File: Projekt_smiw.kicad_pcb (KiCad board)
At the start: 4 copper layers, 53 x 33 mm, 24 parts, among them J1 USB_C_Receptacle_USB2.0, J2 Conn_01x08, J3 Conn_01x10, SW1 SW_Omron_B3FS, SW2 SW_Omron_B3FS, U1 USBLC6-2P6, U2 NCP1117-3.3_SOT223, U4 ESP32-S3-PICO-1

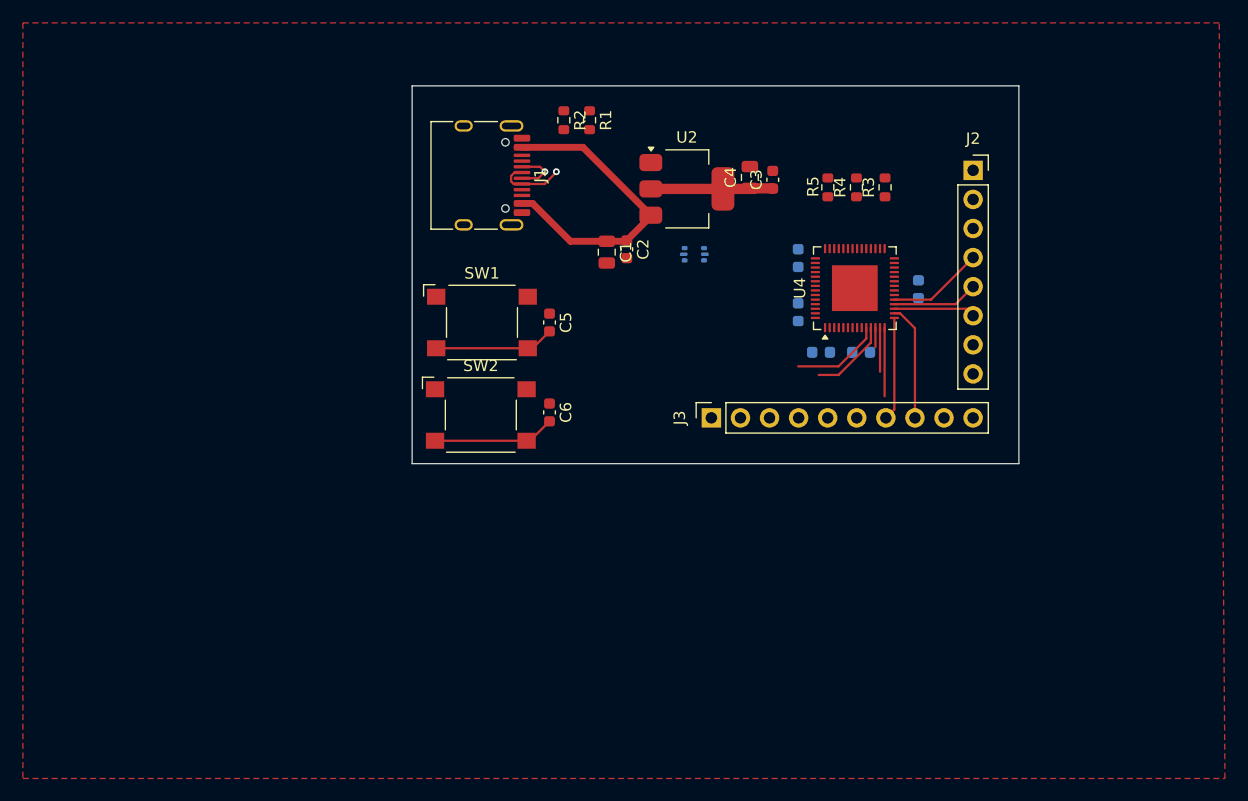
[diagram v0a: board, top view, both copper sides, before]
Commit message: pvcv1
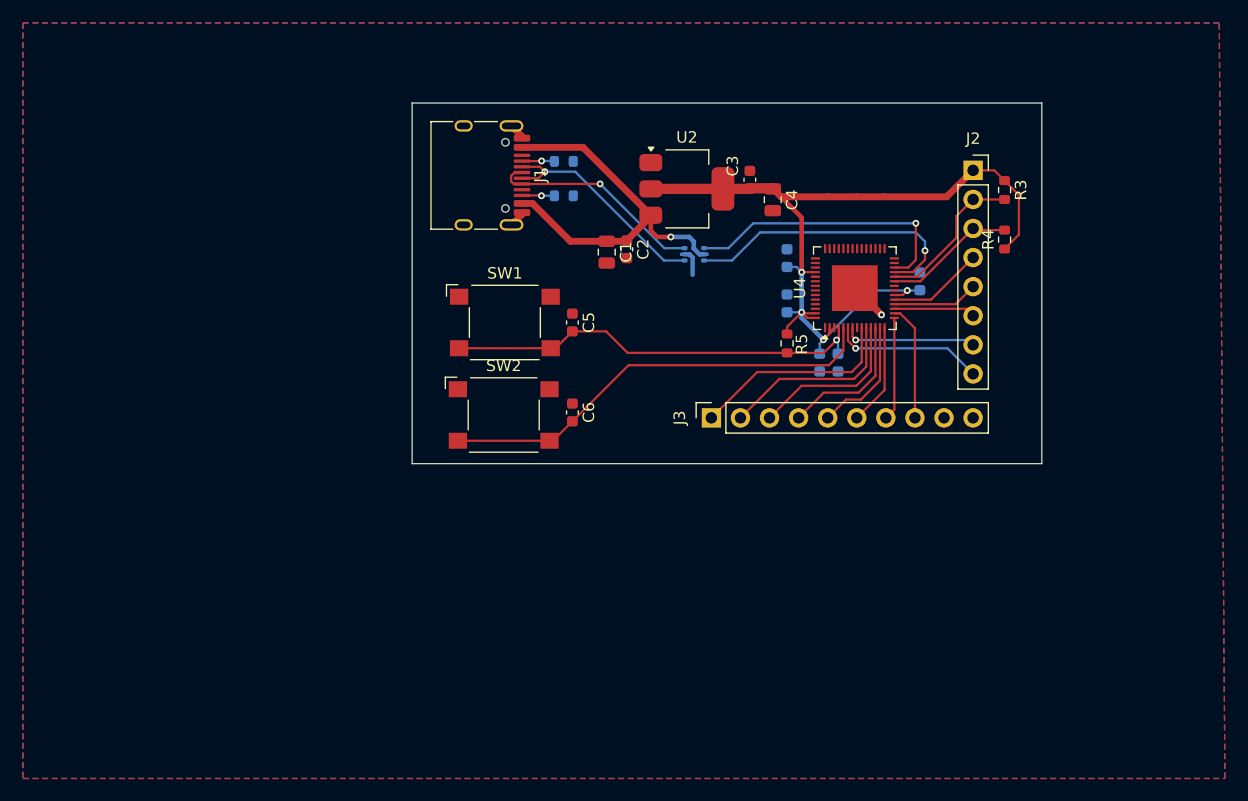
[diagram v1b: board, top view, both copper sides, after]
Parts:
- R1, R2: moved to B.Cu
- moved R5 14.1 mm to (195.8, 62.5), turned to -90 degrees
- moved R4 13.7 mm to (214.8, 53.4)
- moved R3 10.4 mm to (214.8, 49.1), turned to -90 degrees
- moved R1 6.97 mm to (176.2, 49.6), turned to 180 degrees
- moved R2 3.60 mm to (176.2, 46.6), turned to 180 degrees
- moved C4 2.79 mm to (194.5, 50.0), turned to -90 degrees
- moved C7 2.21 mm to (200.2, 64.2), turned to 90 degrees
- moved C3 2.00 mm to (192.5, 48.2)
- moved C5 2.00 mm to (177.0, 60.7)
- moved C6 2.00 mm to (177.0, 68.5)
- moved SW1 2.00 mm to (171.1, 60.7)
- moved SW2 2.00 mm to (171.0, 68.8)
- moved C9 1.24 mm to (195.8, 59.0)
- moved C8 0.97 mm to (195.8, 55.0)
- moved C10 0.91 mm to (198.6, 64.2), turned to -90 degrees
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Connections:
- J2 pad 2: /CS BME280 -> /SCL
- J2 pad 3: /CS FRAM SPI -> /SDA
- J2 pad 7: /SDA -> /CS BME280
- J2 pad 8: /SCL -> /CS FRAM SPI
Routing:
- net +3.3V: track 10.7 -> 77.3 mm, vias 0 -> 4
- net /BOOT: track 10.7 -> 38.9 mm
- net /RESET: track 10.5 -> 37.2 mm, vias 0 -> 1
- net /USB D-: track 0.00 -> 25.4 mm, vias 0 -> 1
- net /USB D+: track 0.00 -> 24.8 mm, vias 0 -> 1
- net /COL 1: track 0.00 -> 18.2 mm
- net /D-: track 4.42 -> 19.8 mm
- net /SCL: track 0.00 -> 13.5 mm
- net /CS FRAM SPI: track 0.00 -> 13.3 mm, vias 0 -> 1
- net /D+: track 6.07 -> 19.1 mm
- net /CS BME280: track 0.00 -> 11.6 mm, vias 0 -> 1
- net /SDA: track 0.00 -> 11.6 mm
- net /COL 4: track 1.71 -> 12.4 mm
- net GND: track 0.00 -> 8.59 mm, vias 0 -> 1
- net /COL 2: track 7.91 -> 16.3 mm
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- added copper zone on B.Cu, net GND
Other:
- board size 53 x 33 mm -> 55 x 31.5 mm

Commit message: Zmianakonnektorav3
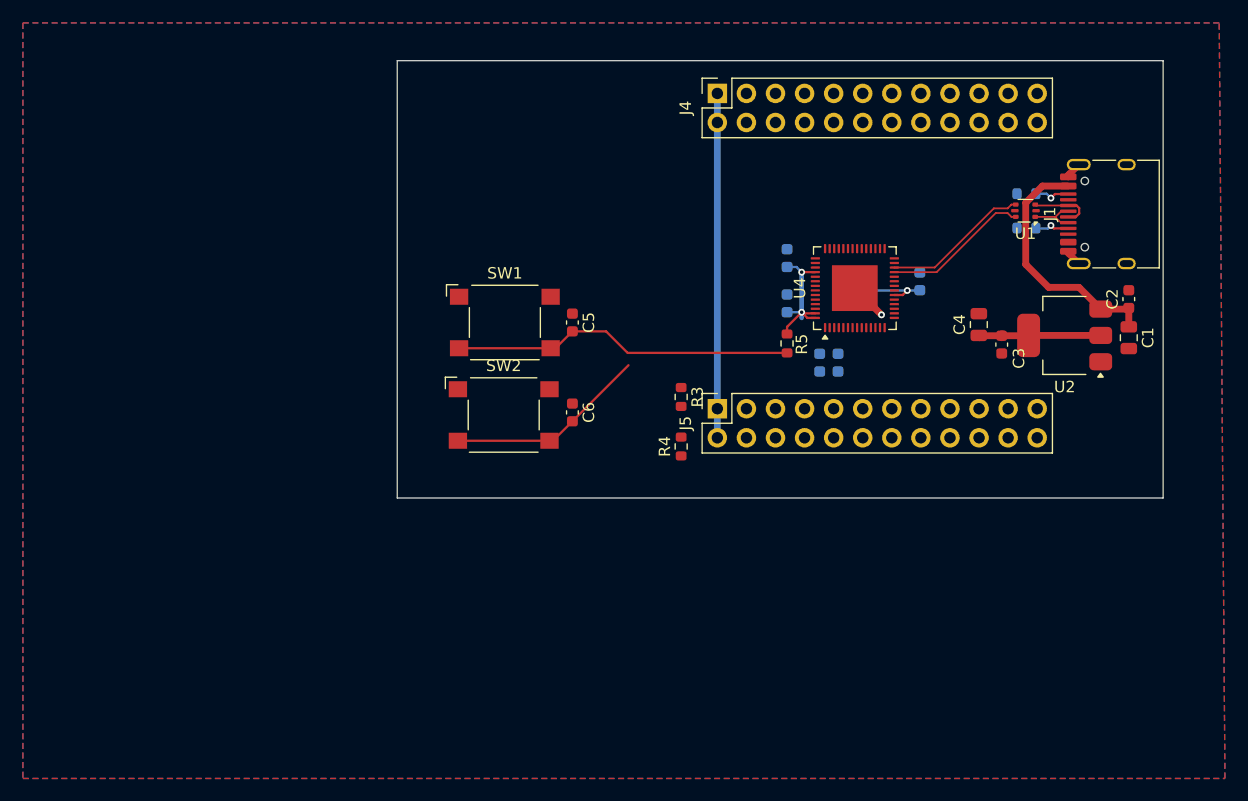
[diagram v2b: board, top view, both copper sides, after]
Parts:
- removed J2: Conn_01x08, Connector_PinSocket_2.54mm:PinSocket_1x08_P2.54mm_Vertical
- removed J3: Conn_01x10, Connector_PinSocket_2.54mm:PinSocket_1x10_P2.54mm_Vertical
- added J4: Conn_02x12_Odd_Even, Connector_PinSocket_2.54mm:PinSocket_2x12_P2.54mm_Vertical, F.Cu at (189.7, 40.7)
- added J5: Conn_02x12_Odd_Even, Connector_PinSocket_2.54mm:PinSocket_2x12_P2.54mm_Vertical, F.Cu at (189.7, 68.2)
- U1: moved to F.Cu
- moved J1 55.9 mm to (224.4, 51.2), turned to 90 degrees
- moved C1 46.2 mm to (225.6, 62.0)
- moved C2 44.1 mm to (225.6, 58.6), turned to 90 degrees
- moved R2 40.8 mm to (216.7, 52.4), turned to 0 degrees
- moved R1 40.4 mm to (216.7, 49.4), turned to 0 degrees
- moved U2 35.4 mm to (220.0, 61.8), turned to 180 degrees
- moved R3 33.5 mm to (186.5, 67.2)
- moved R4 33.5 mm to (186.5, 71.5)
- moved U1 29.2 mm to (216.6, 50.9), turned to 180 degrees
- moved C3 26.3 mm to (214.5, 62.6), turned to -90 degrees
- moved C4 21.0 mm to (212.5, 60.9), turned to 90 degrees
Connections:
- U4 pad 21: unconnected-(U4-XTAL_32K_P-Pad21) -> /XTAL_32K_P
- U4 pad 22: unconnected-(U4-XTAL_32K_N-Pad22) -> /XTAL_32K_N
- U4 pad 27: unconnected-(U4-GPIO21-Pad27) -> /GPIO21
- U4 pad 36: unconnected-(U4-SPICLK_N-Pad36) -> /SPICLK_N
- U4 pad 37: unconnected-(U4-SPICLK_P-Pad37) -> /SPICLK_P
- U4 pad 38: unconnected-(U4-GPIO33-Pad38) -> /GPIO33
- U4 pad 39: unconnected-(U4-GPIO34-Pad39) -> /GPIO34
- U4 pad 40: unconnected-(U4-GPIO35-Pad40) -> /GPIO35
- U4 pad 41: unconnected-(U4-GPIO36-Pad41) -> /GPIO36
- U4 pad 42: unconnected-(U4-GPIO37-Pad42) -> /GPIO37
- U4 pad 43: unconnected-(U4-GPIO38-Pad43) -> /GPIO38
- U4 pad 44: unconnected-(U4-MTCK-Pad44) -> /MTCK
- U4 pad 45: unconnected-(U4-MTDO-Pad45) -> /MTDO
- U4 pad 47: unconnected-(U4-MTDI-Pad47) -> /MTDI
- U4 pad 48: unconnected-(U4-MTMS-Pad48) -> /MTMS
- U4 pad 49: unconnected-(U4-U0TXD-Pad49) -> /UOTXD
- U4 pad 50: unconnected-(U4-U0RXD-Pad50) -> /UORXD
- U4 pad 51: unconnected-(U4-GPIO45-Pad51) -> /GPIO45
- U4 pad 52: unconnected-(U4-GPIO46-Pad52) -> /GPIO46
- U4 pad 8: unconnected-(U4-GPIO3-Pad8) -> /GPIO3
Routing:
- net /BOOT: track 38.9 -> 17.6 mm
- net /COL 1: track 18.2 -> 0.00 mm
- net +3.3V: track 77.3 -> 59.3 mm, vias 4 -> 3
- net /COL 2: track 16.3 -> 0.00 mm
- net /D-: track 19.8 -> 4.45 mm, vias 1 -> 0
- net /COL 3: track 14.3 -> 0.00 mm
- net /D+: track 19.1 -> 5.52 mm, vias 1 -> 0
- net /SCL: track 13.5 -> 0.00 mm
- net /CS FRAM SPI: track 13.3 -> 0.00 mm, vias 1 -> 0
- net +5V: track 34.6 -> 22.1 mm, vias 1 -> 0
- net /USB D-: track 25.4 -> 12.9 mm, vias 1 -> 0
- net /COL 4: track 12.4 -> 0.00 mm
- net /USB D+: track 24.8 -> 12.9 mm, vias 1 -> 0
- net /CS BME280: track 11.6 -> 0.00 mm, vias 1 -> 0
- net /SDA: track 11.6 -> 0.00 mm
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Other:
- board size 55 x 31.5 mm -> 66.9 x 38.2 mm
